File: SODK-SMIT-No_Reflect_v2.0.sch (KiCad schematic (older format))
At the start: 149 parts

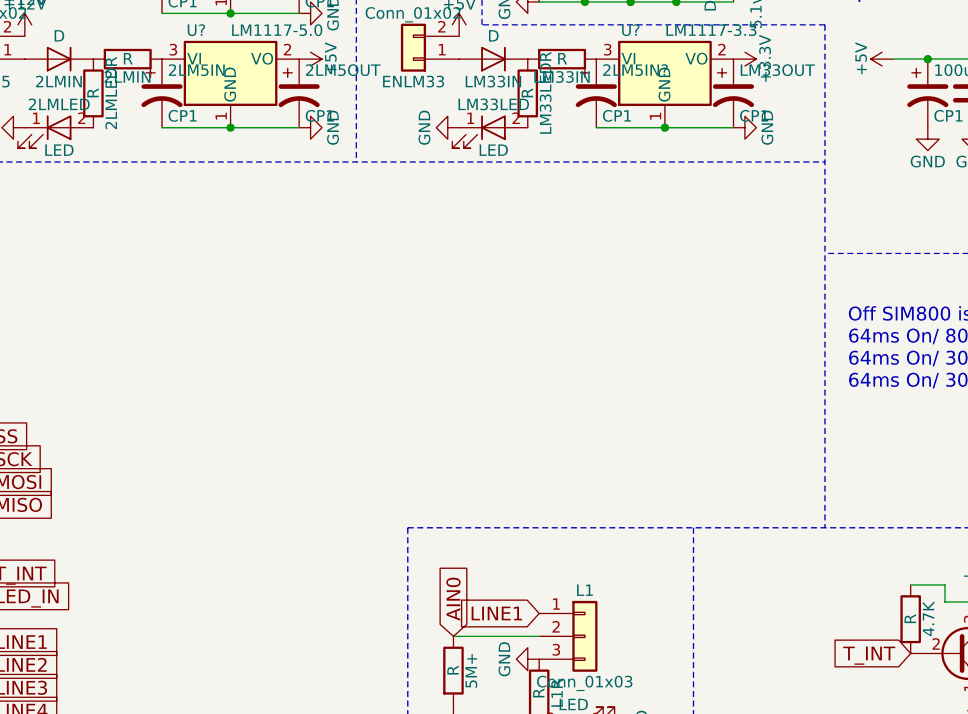
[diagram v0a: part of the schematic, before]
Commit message: 123
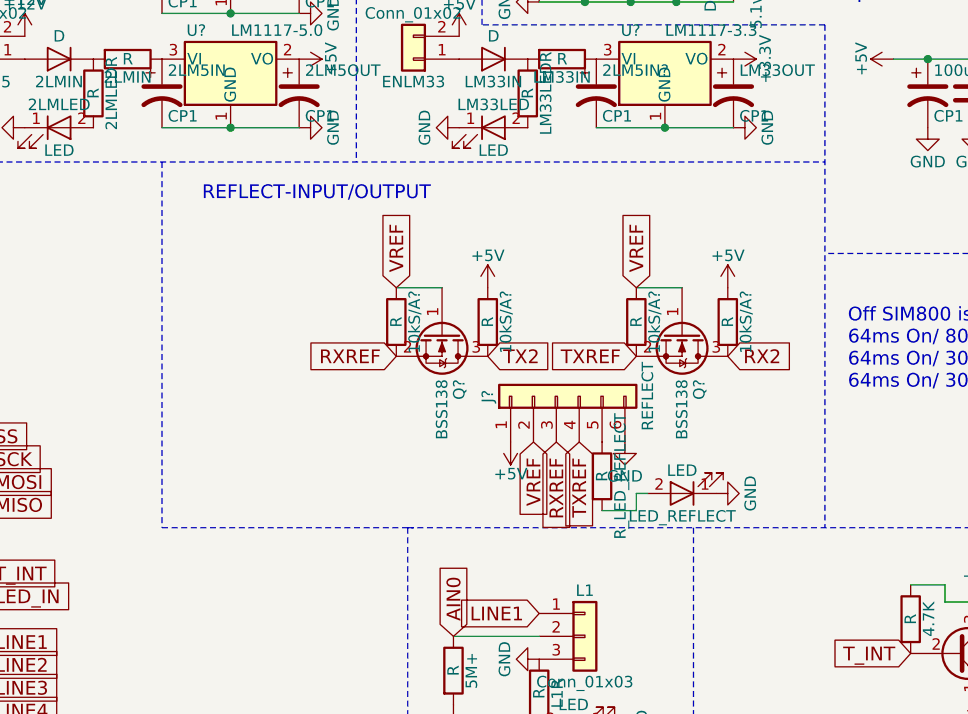
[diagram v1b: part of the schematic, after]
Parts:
- added 10kS/A? (x4), R_LED_REFLECT: R, symbol R
- added J?: REFLECT, symbol Conn_01x06
- added LED_REFLECT: LED, symbol LED
- added Q? (x2): BSS138, TO_SOT_Packages_SMD:SOT-23, symbol BSS138
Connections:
- net +5V: now also 10kS/A?.1, 10kS/A?.1, J?.1 (Pin_1)
- net GND: now also J?.6 (Pin_6), LED_REFLECT.1 (K)
- net RX2: now also 10kS/A?.2, Q?.3 (D)
- net TX2: now also 10kS/A?.2, Q?.3 (D)
- new net: J?.5 (Pin_5), R_LED_REFLECT.1
- new net: LED_REFLECT.2 (A), R_LED_REFLECT.2
- new net RXREF: 10kS/A?.2, J?.3 (Pin_3), Q?.2 (S)
- new net TXREF: 10kS/A?.2, J?.4 (Pin_4), Q?.2 (S)
- new net VREF: 10kS/A?.1, 10kS/A?.1, J?.2 (Pin_2), Q?.1 (G), Q?.1 (G)
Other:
- note added: "REFLECT-INPUT/OUTPUT\n"
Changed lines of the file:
@@
 Text GLabel 5150 3800 2    60   Input ~ 0
 T_INT
+$Comp
+L BSS138 Q?
+U 1 1 5A8EFF44
+P 8225 2750
+F 0 "Q?" H 8425 2825 50  0000 L CNN
+F 1 "BSS138" H 8425 2750 50  0000 L CNN
+F 2 "TO_SOT_Packages_SMD:SOT-23" H 8425 2675 50  0001 L CIN
+F 3 "" H 8225 2750 50  0001 L CNN
+	1    8225 2750
+	0    1    1    0
+$EndComp
+$Comp
+L +5V #PWR?
+U 1 1 5A8EFF4A
+P 8425 2550
+F 0 "#PWR?" H 8425 2400 50  0001 C CNN
+F 1 "+5V" H 8425 2690 50  0000 C CNN
+F 2 "" H 8425 2550 50  0001 C CNN
+F 3 "" H 8425 2550 50  0001 C CNN
+	1    8425 2550
+	1    0    0    -1
+$EndComp
+$Comp
+L R 10kS/A?
+U 1 1 5A8EFF50
+P 8425 2700
+F 0 "10kS/A?" V 8505 2700 50  0000 C CNN
+F 1 "R" V 8425 2700 50  0000 C CNN
+F 2 "" V 8355 2700 50  0001 C CNN
+F 3 "" H 8425 2700 50  0001 C CNN
+	1    8425 2700
+	1    0    0    -1
+$EndComp
+Text GLabel 8025 2550 1    60   Input ~ 0
+VREF
+$Comp
+L R 10kS/A?
+U 1 1 5A8EFF57
+P 8025 2700
+F 0 "10kS/A?" V 8105 2700 50  0000 C CNN
+F 1 "R" V 8025 2700 50  0000 C CNN
+F 2 "" V 7955 2700 50  0001 C CNN
+F 3 "" H 8025 2700 50  0001 C CNN
+	1    8025 2700
+	1    0    0    -1
+$EndComp
+Text GLabel 8425 2850 2    60   Input ~ 0
+RX2
+Text GLabel 8025 2850 0    60   Input ~ 0
+TXREF
+Wire Wire Line
+	8225 2550 8025 2550
+$Comp
+L BSS138 Q?
+U 1 1 5A8F0766
+P 7175 2750
+F 0 "Q?" H 7375 2825 50  0000 L CNN
+F 1 "BSS138" H 7375 2750 50  0000 L CNN
+F 2 "TO_SOT_Packages_SMD:SOT-23" H 7375 2675 50  0001 L CIN
+F 3 "" H 7175 2750 50  0001 L CNN
+	1    7175 2750
+	0    1    1    0
+$EndComp
+$Comp
+L +5V #PWR?
+U 1 1 5A8F076C
+P 7375 2550
+F 0 "#PWR?" H 7375 2400 50  0001 C CNN
+F 1 "+5V" H 7375 2690 50  0000 C CNN
+F 2 "" H 7375 2550 50  0001 C CNN
+F 3 "" H 7375 2550 50  0001 C CNN
+	1    7375 2550
+	1    0    0    -1
+$EndComp
+$Comp
+L R 10kS/A?
+U 1 1 5A8F0772
+P 7375 2700
+F 0 "10kS/A?" V 7455 2700 50  0000 C CNN
+F 1 "R" V 7375 2700 50  0000 C CNN
+F 2 "" V 7305 2700 50  0001 C CNN
+F 3 "" H 7375 2700 50  0001 C CNN
+	1    7375 2700
+	1    0    0    -1
+$EndComp
+Text GLabel 6975 2550 1    60   Input ~ 0
+VREF
+$Comp
+L R 10kS/A?
+U 1 1 5A8F0779
+P 6975 2700
+F 0 "10kS/A?" V 7055 2700 50  0000 C CNN
+F 1 "R" V 6975 2700 50  0000 C CNN
+F 2 "" V 6905 2700 50  0001 C CNN
+F 3 "" H 6975 2700 50  0001 C CNN
+	1    6975 2700
+	1    0    0    -1
+$EndComp
+Text GLabel 7375 2850 2    60   Input ~ 0
+TX2
+Text GLabel 6975 2850 0    60   Input ~ 0
+RXREF
+Wire Wire Line
+	7175 2550 6975 2550
+$Comp
+L Conn_01x06 J?
+U 1 1 5A8F1000
+P 7675 3025
+F 0 "J?" H 7675 3325 50  0000 C CNN
+F 1 "REFLECT" H 7675 2625 50  0000 C CNN
+F 2 "" H 7675 3025 50  0001 C CNN
+F 3 "" H 7675 3025 50  0001 C CNN
+	1    7675 3025
+	0    -1   -1   0
+$EndComp
+$Comp
+L +5V #PWR?
+U 1 1 5A8F1AEC
+P 7475 3225
+F 0 "#PWR?" H 7475 3075 50  0001 C CNN
+F 1 "+5V" H 7475 3365 50  0000 C CNN
+F 2 "" H 7475 3225 50  0001 C CNN
+F 3 "" H 7475 3225 50  0001 C CNN
+	1    7475 3225
+	-1   0    0    1
+$EndComp
+Text GLabel 7575 3225 3    60   Input ~ 0
+VREF
+Text GLabel 7675 3225 3    60   Input ~ 0
+RXREF
+Text GLabel 7775 3225 3    60   Input ~ 0
+TXREF
+$Comp
+L GND #PWR?
+U 1 1 5A8F21B7
+P 7975 3225
+F 0 "#PWR?" H 7975 2975 50  0001 C CNN
+F 1 "GND" H 7975 3075 50  0000 C CNN
+F 2 "" H 7975 3225 50  0001 C CNN
+F 3 "" H 7975 3225 50  0001 C CNN
+	1    7975 3225
+	1    0    0    -1
+$EndComp
+$Comp
+L LED LED_REFLECT
+U 1 1 5A8F2303
+P 8225 3450
+F 0 "LED_REFLECT" H 8225 3550 50  0000 C CNN
+F 1 "LED" H 8225 3350 50  0000 C CNN
+F 2 "" H 8225 3450 50  0001 C CNN
+F 3 "" H 8225 3450 50  0001 C CNN
+	1    8225 3450
+	-1   0    0    1
+$EndComp
+$Comp
+L R R_LED_REFLECT
+U 1 1 5A8F24A0
+P 7875 3375
+F 0 "R_LED_REFLECT" V 7955 3375 50  0000 C CNN
+F 1 "R" V 7875 3375 50  0000 C CNN
+F 2 "" V 7805 3375 50  0001 C CNN
+F 3 "" H 7875 3375 50  0001 C CNN
+	1    7875 3375
+	1    0    0    -1
+$EndComp
+Wire Wire Line
+	7875 3525 8025 3525
+Wire Wire Line
+	8025 3525 8025 3450
+Wire Wire Line
+	8025 3450 8075 3450
+$Comp
+L GND #PWR?
+U 1 1 5A8F28CE
+P 8375 3450
+F 0 "#PWR?" H 8375 3200 50  0001 C CNN
+F 1 "GND" H 8375 3300 50  0000 C CNN
+F 2 "" H 8375 3450 50  0001 C CNN
+F 3 "" H 8375 3450 50  0001 C CNN
+	1    8375 3450
+	0    -1   -1   0
+$EndComp
+Wire Notes Line
+	5950 2000 5950 3600
+Wire Notes Line
+	5950 3600 7050 3600
+Text Notes 6125 2175 0    60   ~ 0
+REFLECT-INPUT/OUTPUT\n
 $EndSCHEMATC
